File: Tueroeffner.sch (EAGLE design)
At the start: 34 parts, among them IC1 NCP1117ST33T3G, IC3 M25PE20, K1 EC2-12SNU, Q1 2N7002CK, Q3 2N7002CK

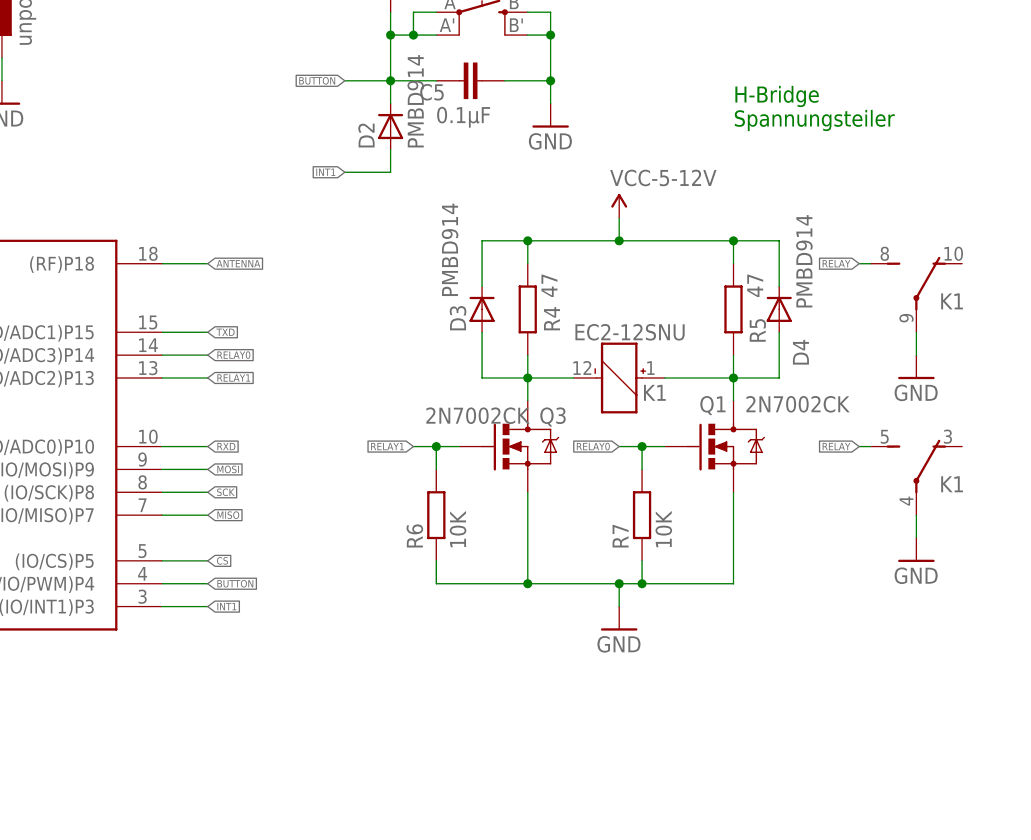
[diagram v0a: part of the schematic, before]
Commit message: New H-Bridge
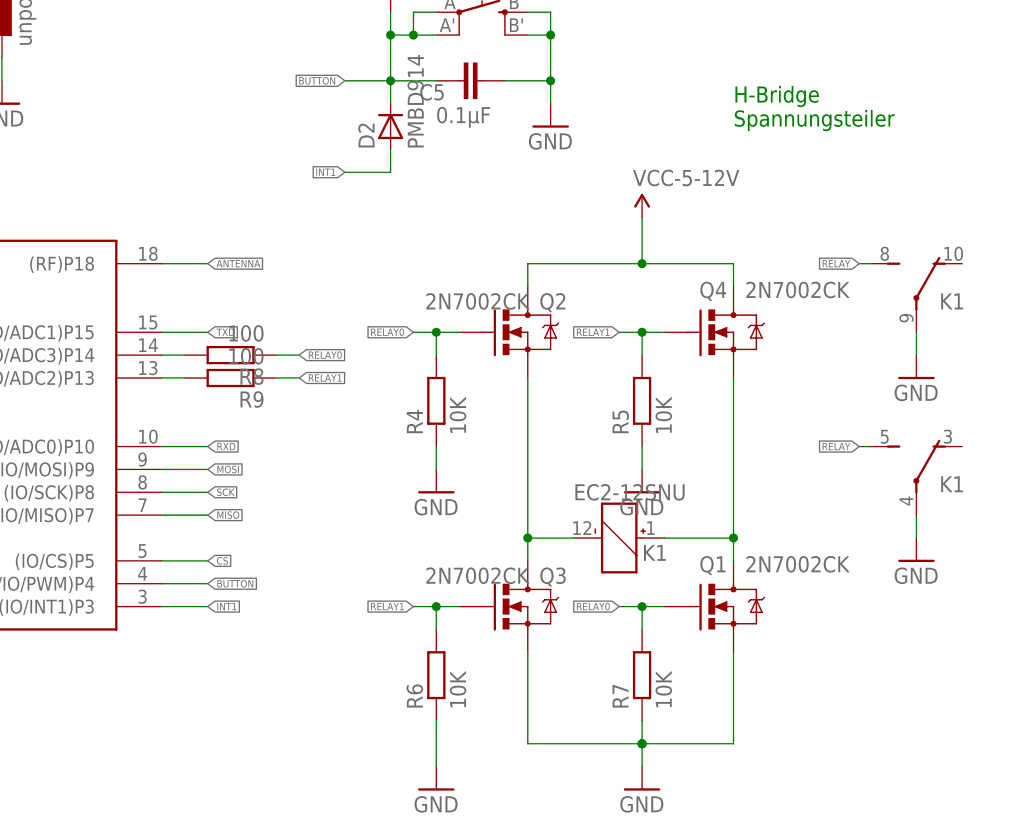
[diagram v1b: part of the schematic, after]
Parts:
- removed D3, D4: PMBD914, semicon-smd-ipc:D-A1-C3
- added Q2, Q4: 2N7002CK, SparkFun-DiscreteSemi:MOSFET-NCHANNELBSS123LT1G
- added R8, R9: 100, resistor:R-EU_M2012
- R4, R5: value 47 -> 10K
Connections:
- new net N$4: R8.2, U$5.(ZEROX/IO/ADC3)P14
- new net N$5: R9.2, U$5.(TRIAC/IO/ADC2)P13
- net DC_5-12V: now also Q2.D, Q4.D; no longer D3.C, D4.C, R4.2, R5.2
- net GND: now also R4.1, R5.1
- net N$2: now also Q2.S; no longer D3.A, R4.1
- net N$3: now also Q4.S; no longer D4.A, R5.1
- net RELAY0: now also Q2.G, R4.2, R8.1; no longer U$5.(ZEROX/IO/ADC3)P14
- net RELAY1: now also Q4.G, R5.2, R9.1; no longer U$5.(TRIAC/IO/ADC2)P13
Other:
- moved on the sheet: K1, Q1, Q3, R4, R5, R6, R7

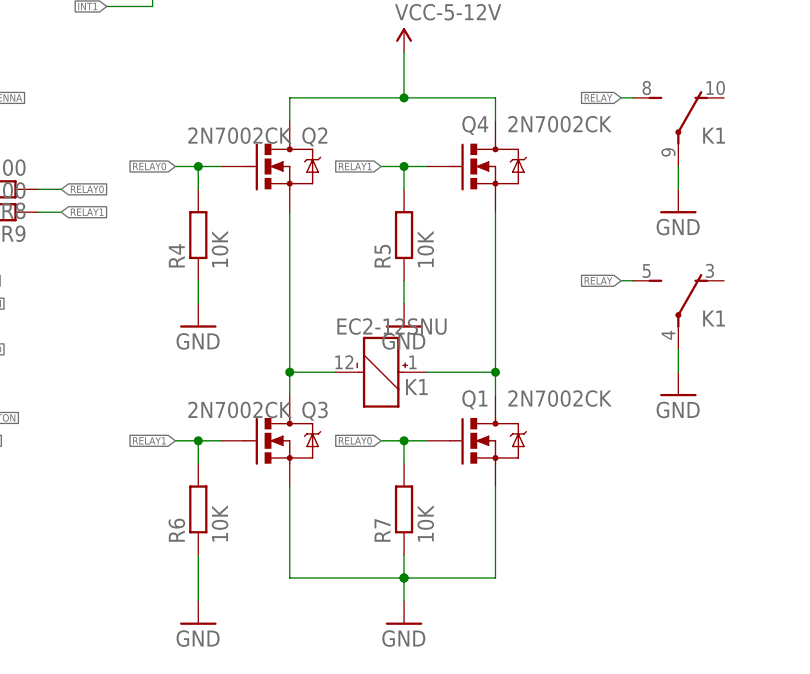
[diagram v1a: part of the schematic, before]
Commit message: Basic Routing
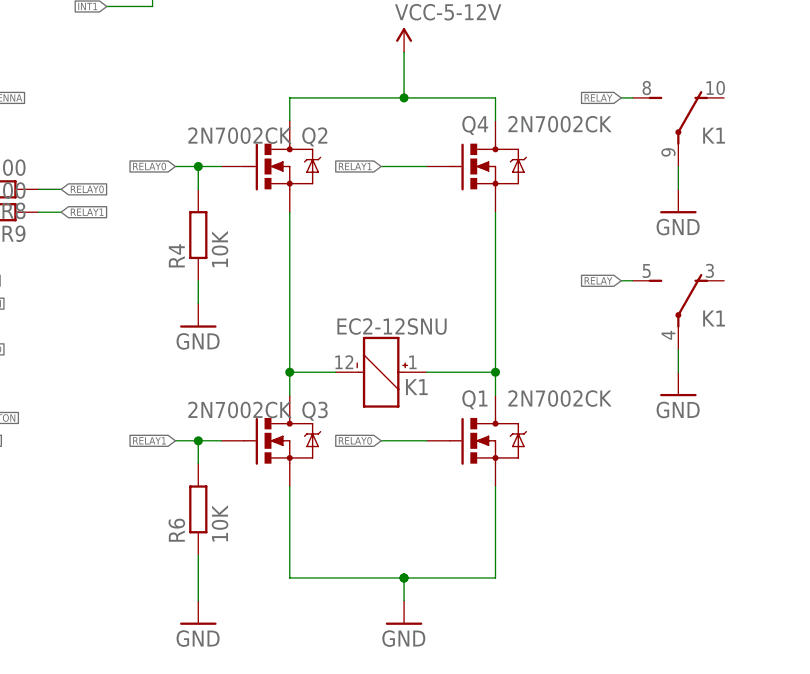
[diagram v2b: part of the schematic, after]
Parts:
- removed R5, R7: 10K, resistor:R-EU_M2012
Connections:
- net GND: no longer R5.1, R7.1
- net RELAY0: no longer R7.2
- net RELAY1: no longer R5.2
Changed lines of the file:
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@@
 <part name="B1" library="rectifier" deviceset="RECTIFIER-" device="S40"/>
 <part name="R6" library="resistor" deviceset="R-EU_" device="M2012" value="10K"/>
-<part name="R7" library="resistor" deviceset="R-EU_" device="M2012" value="10K"/>
 <part name="Q3" library="SparkFun-DiscreteSemi" deviceset="MOSFET-NCHANNEL" device="BSS123LT1G" value="2N7002CK"/>
 <part name="Q1" library="SparkFun-DiscreteSemi" deviceset="MOSFET-NCHANNEL" device="BSS123LT1G" value="2N7002CK"/>
@@
 <part name="JP3" library="SparkFun-Connectors" deviceset="M04" device="SCREW"/>
 <part name="R4" library="resistor" deviceset="R-EU_" device="M2012" value="10K"/>
-<part name="R5" library="resistor" deviceset="R-EU_" device="M2012" value="10K"/>
 <part name="Q2" library="SparkFun-DiscreteSemi" deviceset="MOSFET-NCHANNEL" device="BSS123LT1G" value="2N7002CK"/>
 <part name="Q4" library="SparkFun-DiscreteSemi" deviceset="MOSFET-NCHANNEL" device="BSS123LT1G" value="2N7002CK"/>
 <part name="GND8" library="supply1" deviceset="GND" device=""/>
-<part name="GND9" library="supply1" deviceset="GND" device=""/>
 <part name="GND10" library="supply1" deviceset="GND" device=""/>
 <part name="R8" library="resistor" deviceset="R-EU_" device="M2012" value="100"/>
@@
 <attribute name="VALUE" x="262.382" y="-6.35" size="1.778" layer="96" rot="R90"/>
 </instance>
-<instance part="R7" gate="G$1" x="281.94" y="-2.54" smashed="yes" rot="R90">
-<attribute name="NAME" x="280.4414" y="-6.35" size="1.778" layer="95" rot="R90"/>
-<attribute name="VALUE" x="285.242" y="-6.35" size="1.778" layer="96" rot="R90"/>
-</instance>
 <instance part="Q3" gate="G$1" x="269.24" y="5.08" smashed="yes">
 <attribute name="NAME" x="270.51" y="7.62" size="1.778" layer="95"/>
@@
 <attribute name="VALUE" x="262.382" y="24.13" size="1.778" layer="96" rot="R90"/>
 </instance>
-<instance part="R5" gate="G$1" x="281.94" y="27.94" smashed="yes" rot="R90">
-<attribute name="NAME" x="280.4414" y="24.13" size="1.778" layer="95" rot="R90"/>
-<attribute name="VALUE" x="285.242" y="24.13" size="1.778" layer="96" rot="R90"/>
-</instance>
 <instance part="Q2" gate="G$1" x="269.24" y="35.56" smashed="yes">
 <attribute name="NAME" x="270.51" y="38.1" size="1.778" layer="95"/>
@@
 <instance part="GND8" gate="1" x="259.08" y="17.78" smashed="yes">
 <attribute name="VALUE" x="256.54" y="15.24" size="1.778" layer="96"/>
-</instance>
-<instance part="GND9" gate="1" x="281.94" y="17.78" smashed="yes">
-<attribute name="VALUE" x="279.4" y="15.24" size="1.778" layer="96"/>
 </instance>
 <instance part="GND10" gate="1" x="259.08" y="-15.24" smashed="yes">
@@
 <wire x1="281.94" y1="-12.7" x2="281.94" y2="-10.16" width="0.1524" layer="91"/>
 <junction x="281.94" y="-10.16"/>
-<pinref part="R7" gate="G$1" pin="1"/>
-<wire x1="281.94" y1="-7.62" x2="281.94" y2="-10.16" width="0.1524" layer="91"/>
 <junction x="281.94" y="-10.16"/>
 <pinref part="Q3" gate="G$1" pin="S"/>
@@
 <pinref part="R4" gate="G$1" pin="1"/>
 <wire x1="259.08" y1="20.32" x2="259.08" y2="22.86" width="0.1524" layer="91"/>
-</segment>
-<segment>
-<pinref part="GND9" gate="1" pin="GND"/>
-<pinref part="R5" gate="G$1" pin="1"/>
-<wire x1="281.94" y1="20.32" x2="281.94" y2="22.86" width="0.1524" layer="91"/>
 </segment>
 <segment>
@@
 </segment>
 <segment>
-<wire x1="284.48" y1="5.08" x2="281.94" y2="5.08" width="0.1524" layer="91"/>
 <label x="279.4" y="5.08" size="0.8128" layer="95" rot="R180" xref="yes"/>
-<pinref part="R7" gate="G$1" pin="2"/>
-<wire x1="281.94" y1="5.08" x2="279.4" y2="5.08" width="0.1524" layer="91"/>
-<wire x1="281.94" y1="2.54" x2="281.94" y2="5.08" width="0.1524" layer="91"/>
-<junction x="281.94" y="5.08"/>
+<wire x1="284.48" y1="5.08" x2="279.4" y2="5.08" width="0.1524" layer="91"/>
 <pinref part="Q1" gate="G$1" pin="G"/>
 </segment>
@@
 </segment>
 <segment>
-<wire x1="284.48" y1="35.56" x2="281.94" y2="35.56" width="0.1524" layer="91"/>
 <label x="279.4" y="35.56" size="0.8128" layer="95" rot="R180" xref="yes"/>
-<pinref part="R5" gate="G$1" pin="2"/>
-<wire x1="281.94" y1="35.56" x2="279.4" y2="35.56" width="0.1524" layer="91"/>
-<wire x1="281.94" y1="33.02" x2="281.94" y2="35.56" width="0.1524" layer="91"/>
-<junction x="281.94" y="35.56"/>
+<wire x1="284.48" y1="35.56" x2="279.4" y2="35.56" width="0.1524" layer="91"/>
 <pinref part="Q4" gate="G$1" pin="G"/>
 </segment>
